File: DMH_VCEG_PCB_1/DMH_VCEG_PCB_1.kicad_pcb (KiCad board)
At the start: 2 copper layers, 148 x 175 mm, 229 parts, among them J1 TS_Jack_6.35mm_Sw, J10 TS_Jack_6.35mm_Sw, J100 IDC_02x08, J11 TS_Jack_6.35mm_Sw, J12 TS_Jack_6.35mm_Sw, J13 TS_Jack_6.35mm_Sw, J14 TS_Jack_6.35mm_Sw, J15 TS_Jack_6.35mm_Sw, J16 TS_Jack_6.35mm_Sw, J17 TS_Jack_6.35mm_Sw, J18 TS_Jack_6.35mm_Sw, J19 TS_Jack_6.35mm_Sw, J2 TS_Jack_6.35mm_Sw, J20 TS_Jack_6.35mm_Sw, J200 IDC_02x08, J21 Conn_01x10_PinHeader, J22 Conn_01x10_PinHeader, J23 Conn_01x10_PinHeader, J24 Conn_01x06_PinHeader, J25 Conn_01x10_PinHeader, J26 Conn_01x10_PinHeader, J27 Conn_01x10_PinHeader, J3 TS_Jack_6.35mm_Sw, J4 TS_Jack_6.35mm_Sw, J5 TS_Jack_6.35mm_Sw, J6 TS_Jack_6.35mm_Sw, J7 TS_Jack_6.35mm_Sw, J8 TS_Jack_6.35mm_Sw, J9 TS_Jack_6.35mm_Sw, Q1 BC558, Q17 BC558, Q18 BC558, Q19 BC548, Q2 BC558, Q20 BC548, Q21 MMBFJ113, Q22 MMBFJ113, Q3 BC548, Q4 BC548, Q5 MMBFJ113, Q6 MMBFJ113, U1 TL074, U11 TL074, U12 4001, U13 40106, U15 TL074, U16 4001, U17 TL074, U2 4001, U3 40106, U5 TL074, U6 4001, U7 TL074

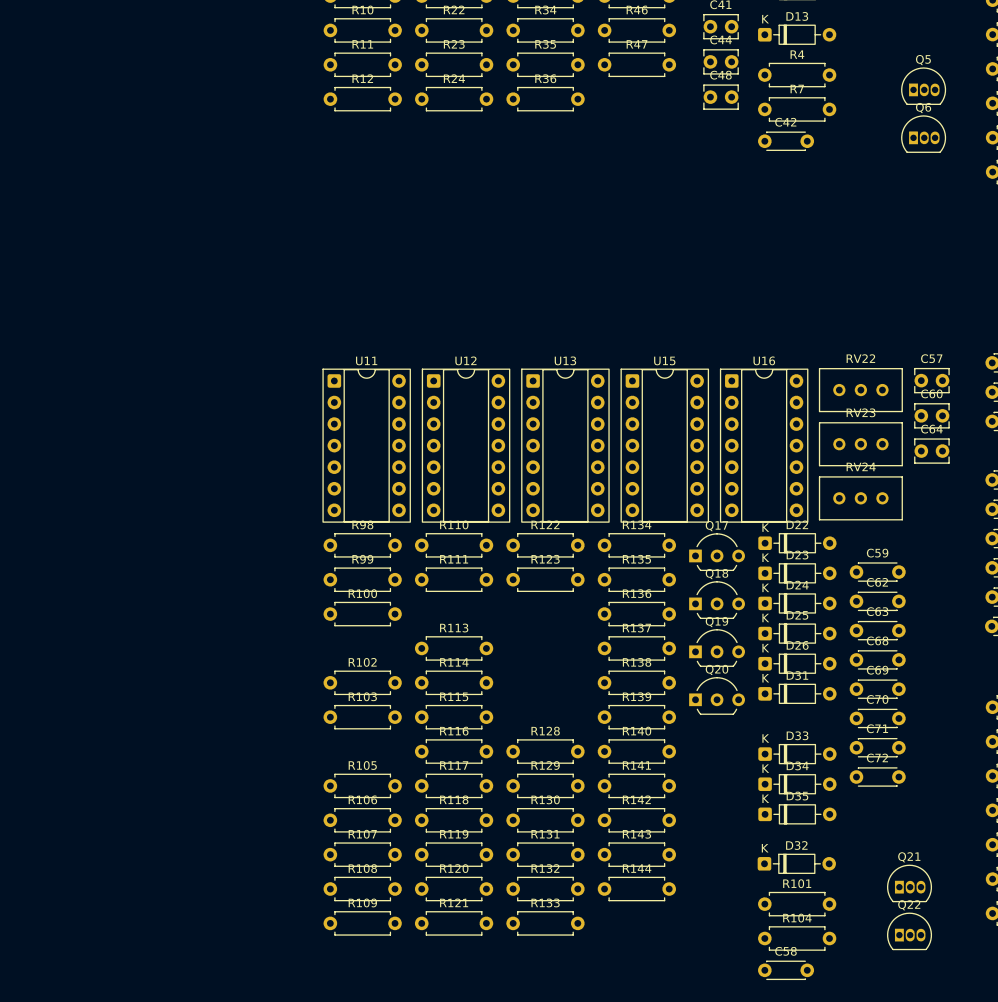
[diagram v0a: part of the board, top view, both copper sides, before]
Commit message: PCB 2 routing in progress
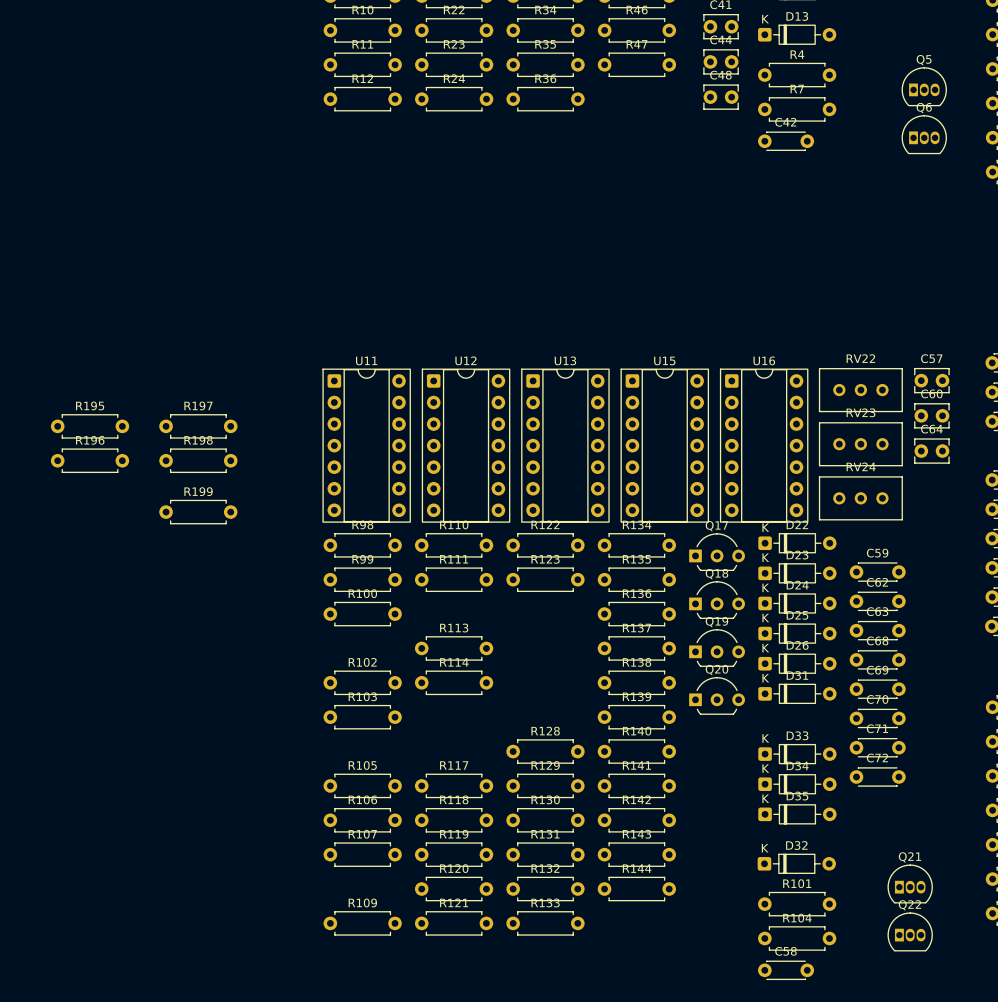
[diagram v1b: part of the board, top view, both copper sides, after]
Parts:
- removed R108, R115, R116: 100k, Resistor_THT:R_Axial_DIN0207_L6.3mm_D2.5mm_P7.62mm_Horizontal
- added R195: 100R, Resistor_THT:R_Axial_DIN0207_L6.3mm_D2.5mm_P7.62mm_Horizontal, F.Cu at (197.4, 139.2)
- added R196: 47k, Resistor_THT:R_Axial_DIN0207_L6.3mm_D2.5mm_P7.62mm_Horizontal, F.Cu at (197.4, 143.2)
- added R197: 68k, Resistor_THT:R_Axial_DIN0207_L6.3mm_D2.5mm_P7.62mm_Horizontal, F.Cu at (210.1, 139.2)
- added R198: 100k, Resistor_THT:R_Axial_DIN0207_L6.3mm_D2.5mm_P7.62mm_Horizontal, F.Cu at (210.1, 143.2)
- added R199: 100R, Resistor_THT:R_Axial_DIN0207_L6.3mm_D2.5mm_P7.62mm_Horizontal, F.Cu at (210.1, 149.2)
- Q21, Q22, Q5, Q6: value MMBFJ113 -> BS170; footprint Package_TO_SOT_THT:TO-92L_Inline -> Package_TO_SOT_THT:TO-92_Inline
- R129, R32: value 100k -> 51k
- R131, R19, R34: value 100k -> 47k
- R18: value 100k -> 68k
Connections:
- C46 pad 1: Net-(D13-K) -> /Core Circuit A/ProcGate
- C48 pad 2: /Core Circuit A/ProcGate -> Net-(D5-A)
- C62 pad 1: Net-(D22-K) -> /Core Circuit B/ProcGate
- C64 pad 2: /Core Circuit B/ProcGate -> Net-(D24-A)
- D22 pad 1: Net-(D22-K) -> /Core Circuit B/ProcGate
- D24 pad 1: Net-(D22-K) -> /Core Circuit B/ProcGate
- D24 pad 2: /Core Circuit B/ProcGate -> Net-(D24-A)
- D3 pad 1: Net-(D13-K) -> /Core Circuit A/ProcGate
- D32 pad 1: Net-(D22-K) -> Net-(D32-K)
- D5 pad 1: Net-(D13-K) -> /Core Circuit A/ProcGate
- D5 pad 2: /Core Circuit A/ProcGate -> Net-(D5-A)
- J21 pad 3: /Core Circuit A/Sus State -> /Core Circuit A/Sus_State
- J22 pad 2: /Core Circuit A/Sus State -> /Core Circuit A/Inv Sus State
- J22 pad 5: unconnected-(J22E-Pin_5-Pad5) -> /CV Processing A/Att CV
- J22 pad 6: unconnected-(J22F-Pin_6-Pad6) -> /CV Processing A/Dec CV
- J22 pad 7: unconnected-(J22G-Pin_7-Pad7) -> /CV Processing A/Sus CV
- J22 pad 8: unconnected-(J22H-Pin_8-Pad8) -> /CV Processing A/Rel CV
- J23 pad 10: /CV Processing A/Rel CV -> unconnected-(J23J-Pin_10-Pad10)
- J23 pad 3: /CV Processing A/Att CV -> unconnected-(J23C-Pin_3-Pad3)
- J23 pad 6: /CV Processing A/Dec CV -> unconnected-(J23F-Pin_6-Pad6)
- J23 pad 7: /CV Processing A/Sus CV -> unconnected-(J23G-Pin_7-Pad7)
- J24 pad 2: Net-(D13-A) -> /Core Circuit A/ProcGate
- J24 pad 3: Net-(J24C-Pin_3) -> Net-(D13-K)
- J24 pad 4: Net-(J24D-Pin_4) -> Net-(D32-K)
- J24 pad 5: Net-(D32-A) -> /Core Circuit B/ProcGate
- J25 pad 3: /Core Circuit B/Sus State -> /Core Circuit B/Sus_State
- J26 pad 2: /Core Circuit B/Sus State -> /Core Circuit B/Inv Sus State
- J26 pad 5: unconnected-(J26E-Pin_5-Pad5) -> /CV Processing B/Att CV
- J26 pad 6: unconnected-(J26F-Pin_6-Pad6) -> /CV Processing B/Dec CV
- J26 pad 7: unconnected-(J26G-Pin_7-Pad7) -> /CV Processing B/Sus CV
- J26 pad 8: unconnected-(J26H-Pin_8-Pad8) -> /CV Processing B/Rel CV
- J27 pad 10: /CV Processing B/Rel CV -> unconnected-(J27J-Pin_10-Pad10)
- J27 pad 3: /CV Processing B/Att CV -> unconnected-(J27C-Pin_3-Pad3)
- J27 pad 6: /CV Processing B/Dec CV -> unconnected-(J27F-Pin_6-Pad6)
- J27 pad 7: /CV Processing B/Sus CV -> unconnected-(J27G-Pin_7-Pad7)
- Q21 pad 1: Net-(Q18-C) -> Net-(J25F-Pin_6)
- Q21 pad 2: Net-(J25F-Pin_6) -> /Core Circuit B/ProcGate
- Q21 pad 3: Net-(Q21-G) -> Net-(Q18-C)
- Q22 pad 1: Net-(Q20-C) -> Net-(J25F-Pin_6)
- Q22 pad 2: Net-(J25F-Pin_6) -> /Core Circuit B/InvGate
- Q22 pad 3: Net-(Q22-G) -> Net-(Q20-C)
- Q5 pad 1: Net-(Q2-C) -> Net-(J21F-Pin_6)
- Q5 pad 2: Net-(J21F-Pin_6) -> /Core Circuit A/ProcGate
- Q5 pad 3: Net-(Q5-G) -> Net-(Q2-C)
- Q6 pad 1: Net-(Q4-C) -> Net-(J21F-Pin_6)
- Q6 pad 2: Net-(J21F-Pin_6) -> /Core Circuit A/InvGate
- Q6 pad 3: Net-(Q6-G) -> Net-(Q4-C)
- R11 pad 1: Net-(Q5-G) -> Net-(R11-Pad1)
- R11 pad 2: /Core Circuit A/ProcGate -> GND
- R120 pad 1: /Core Circuit B/ProcGate -> Net-(D24-A)
- R121 pad 2: Net-(D22-K) -> /Core Circuit B/ProcGate
- R131 pad 1: Net-(J24D-Pin_4) -> Net-(D32-A)
- R134 pad 1: Net-(U15A-+) -> Net-(U15A--)
- R138 pad 1: -12V -> Net-(U15A-+)
- R138 pad 2: Net-(U15A--) -> Net-(D34-A)
- R141 pad 1: Net-(U15A--) -> Net-(U15A-+)
- R18 pad 1: -12V -> +12V
- R18 pad 2: Net-(Q6-G) -> Net-(R11-Pad1)
- R19 pad 1: Net-(Q6-G) -> GND
- R19 pad 2: /Core Circuit A/InvGate -> Net-(U15C--)
- R23 pad 1: /Core Circuit A/ProcGate -> Net-(D5-A)
- R24 pad 2: Net-(D13-K) -> /Core Circuit A/ProcGate
- R34 pad 1: Net-(J24C-Pin_3) -> Net-(D13-A)
- R37 pad 1: Net-(U5A-+) -> Net-(U5A--)
- R41 pad 1: -12V -> Net-(D15-A)
- R41 pad 2: Net-(U5A--) -> Net-(U5A-+)
- R44 pad 1: Net-(U5A--) -> GND
- R44 pad 2: GND -> Net-(U5A-+)
- U1 pad 1: /Core Circuit A/ProcGate -> Net-(D5-A)
- U1 pad 14: Net-(J24C-Pin_3) -> Net-(D13-A)
- U1 pad 8: Net-(U5A-+) -> Net-(U5A--)
- U11 pad 1: /Core Circuit B/ProcGate -> Net-(D24-A)
- U11 pad 14: Net-(J24D-Pin_4) -> Net-(D32-A)
- U11 pad 8: Net-(U15A-+) -> Net-(U15A--)
- U13 pad 1: Net-(D22-K) -> /Core Circuit B/ProcGate
- U13 pad 4: Net-(U13-Pad4) -> Net-(D35-A)
- U13 pad 8: unconnected-(U13-Pad8) -> Net-(U13-Pad8)
- U13 pad 9: GND -> Net-(C71-Pad2)
- U15 pad 9: /CV Processing B/Max Level -> Net-(U15C--)
- U16 pad 10: Net-(D35-A) -> Net-(U16-Pad10)
- U16 pad 13: /Core Circuit B/Sus State -> /Core Circuit B/Sus_State
- U16 pad 2: Net-(U16-Pad2) -> /Core Circuit B/Inv Sus State
- U16 pad 3: /Core Circuit B/Sus State -> /Core Circuit B/Sus_State
- U16 pad 4: Net-(U16-Pad2) -> /Core Circuit B/Inv Sus State
- U16 pad 5: /Core Circuit B/Sus State -> /Core Circuit B/Sus_State
- U16 pad 6: Net-(C71-Pad2) -> Net-(U16-Pad10)
- U16 pad 9: Net-(U13-Pad4) -> Net-(U13-Pad8)
- U3 pad 1: Net-(D13-K) -> /Core Circuit A/ProcGate
- U3 pad 4: Net-(U3-Pad4) -> Net-(D16-A)
- U3 pad 8: unconnected-(U3-Pad8) -> Net-(U3-Pad8)
- U3 pad 9: GND -> Net-(C55-Pad2)
- U5 pad 9: /CV Processing A/Max Level -> Net-(U5C--)
- U6 pad 10: Net-(D16-A) -> Net-(U6-Pad10)
- U6 pad 13: /Core Circuit A/Sus State -> /Core Circuit A/Sus_State
- U6 pad 2: Net-(U6-Pad2) -> /Core Circuit A/Inv Sus State
- U6 pad 3: /Core Circuit A/Sus State -> /Core Circuit A/Sus_State
- U6 pad 4: Net-(U6-Pad2) -> /Core Circuit A/Inv Sus State
- U6 pad 5: /Core Circuit A/Sus State -> /Core Circuit A/Sus_State
- U6 pad 6: Net-(C55-Pad2) -> Net-(U6-Pad10)
- U6 pad 9: Net-(U3-Pad4) -> Net-(U3-Pad8)
